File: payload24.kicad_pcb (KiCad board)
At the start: 6 copper layers, 87.1 x 89.4 mm, 21 parts, among them J1 532540370, J2 532540370, J3 460150206, J4 532540370, Q1 CSD19503KCS, Q2 CSD19503KCS, SW1 FingerTech

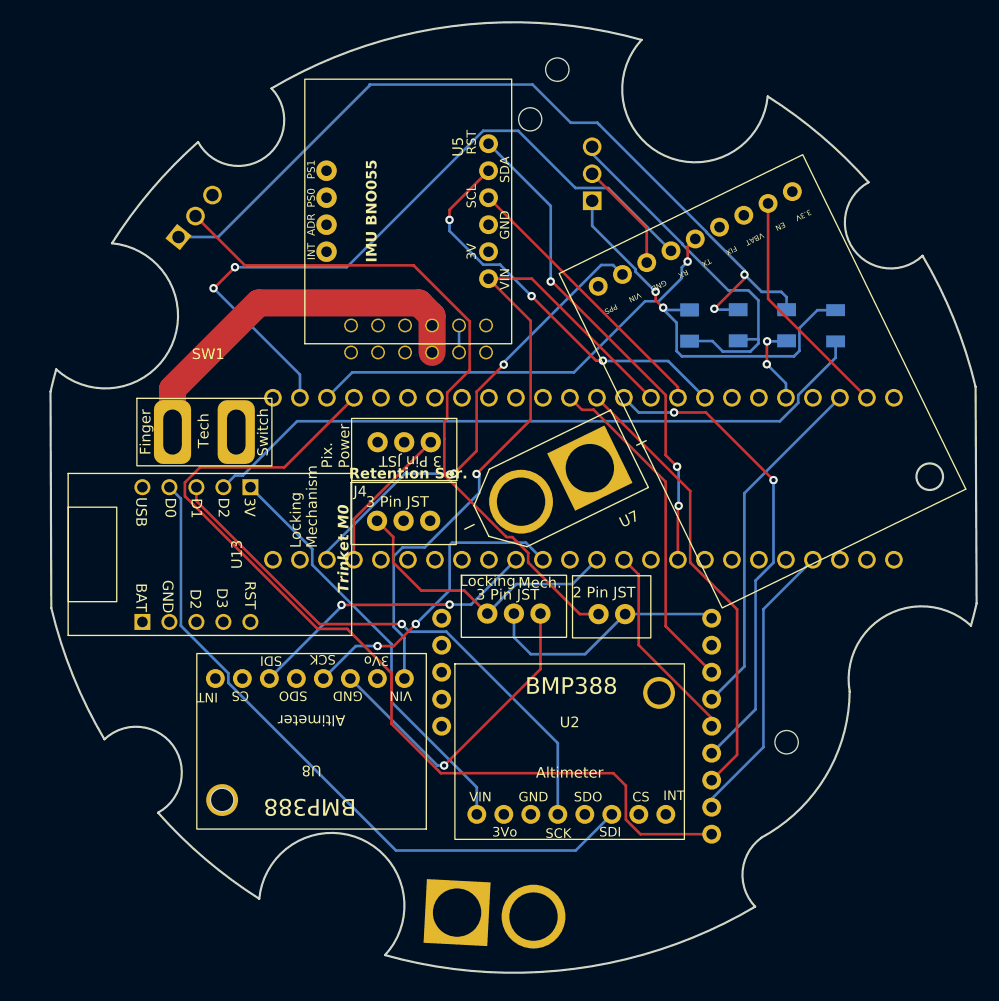
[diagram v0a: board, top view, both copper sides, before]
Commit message: update
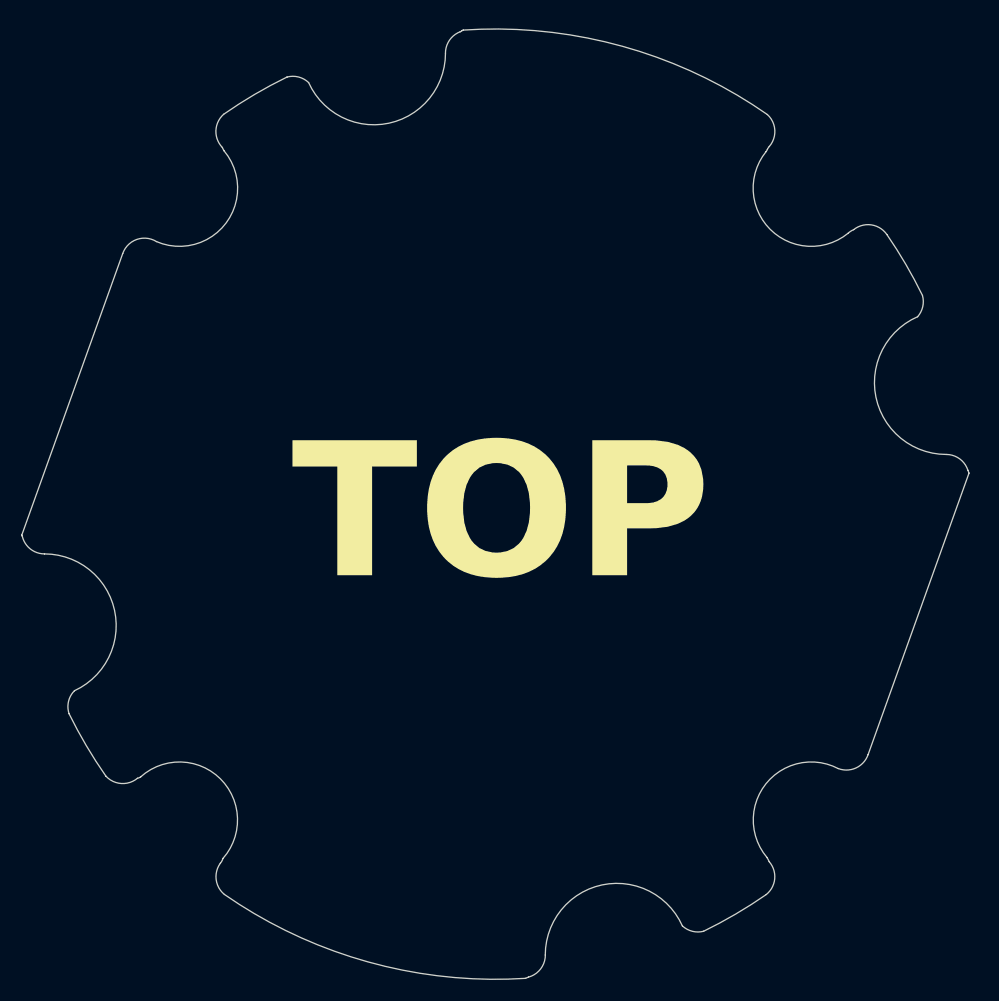
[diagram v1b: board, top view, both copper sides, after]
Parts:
- removed J1, J2, J4: 532540370, JST-XH3:JST-XH3
- removed J3: 460150206, JST-XH2:JST-XH2
- removed Q1, Q2: CSD19503KCS, teensyMosfet:teensyMosfet
- removed R1: 500, 500Ohm:RESC3216X65N
- removed R2: 1000, 1kOhm:RESC3216X70N
- removed R3, R4: 10K, 10KOhm:RESC3216X70N
- removed SW1: FingerTech, FingerTech:FingerTech
- removed U1: ~, Teensy:TEENSY41
- removed U13: ~, Trinket M0:Trinket M0
- removed U14: ~, BNO055:BNO055
- removed U2, U8: ~, BMP388:BMP388
- removed U3: ~, adafruit gps:GPS_adafruit
- removed U4: ~, RFModule:RFM_LoRa
- removed U5: ~, poluluRegulator:VoltageRegulator
- removed U6, U7: ~, XT60:AMASS_XT60-M
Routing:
- net RST3: track 87.9 -> 0.00 mm
- net Net-(Q2-Pad1): track 79.6 -> 0.00 mm, vias 2 -> 0
- net RX1: track 67.5 -> 0.00 mm, vias 2 -> 0
- net 3.3V-Teensy: track 66.4 -> 0.00 mm, vias 1 -> 0
- net GND - NMOS2: track 65.8 -> 0.00 mm
- net SDA3: track 64.7 -> 0.00 mm
- net Power Signal: track 64.6 -> 0.00 mm
- net SCL3: track 51.4 -> 0.00 mm, vias 1 -> 0
- net RST2: track 46.7 -> 0.00 mm, vias 3 -> 0
- net MISO: track 45.4 -> 0.00 mm, vias 2 -> 0
- net 3.3V-Teensy1: track 43.9 -> 0.00 mm, vias 2 -> 0
- net MOSI: track 42.4 -> 0.00 mm
- net TX1: track 42.3 -> 0.00 mm, vias 1 -> 0
- net GND - NMOS1: track 40.7 -> 0.00 mm, vias 1 -> 0
- net 3.3V-Trinket: track 39.6 -> 0.00 mm
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- removed copper zone on In4.Cu, net /22.2V
- removed copper zone on In2.Cu, net 5V-Power Reg.
- removed copper zone on In1.Cu, net GND
- removed copper zone on In3.Cu, net GND - NMOS1
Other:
- board size 87.1 x 89.4 mm -> 89.1 x 89.4 mm
- board text added: "BOTTOM"
- board text added: "TOP"
- board text removed: "Locking"
- board text removed: "Mech."
- board text removed: "Mechanism"
- board text removed: "Pix. Power"
- board text removed: "Retention Ser."

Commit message: PCB laid out
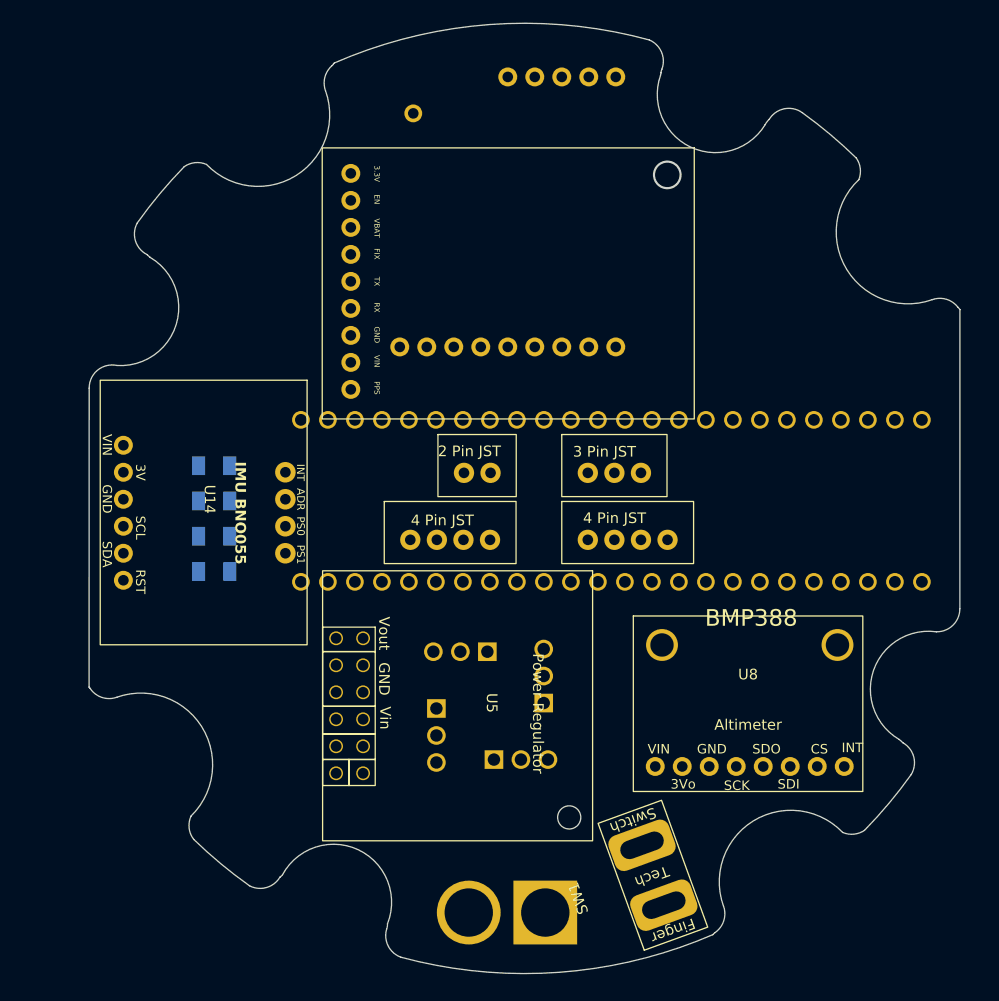
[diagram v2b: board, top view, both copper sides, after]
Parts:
- added J1: JST-XH3, JST-XH3:JST-XH3, F.Cu at (69.2, 54.2)
- added J2: PixHawk, JST-XH2:JST-XH2, F.Cu at (57.5, 54.2)
- added J3: Motors, JST-XH3:JST-XH4, F.Cu at (69.2, 60.5)
- added J4: Motors, JST-XH3:JST-XH4, F.Cu at (52.5, 60.5)
- added Q2: CSD19503KCS, teensyMosfet:teensyMosfet, B.Cu at (59.6, 74.6)
- added Q3: IRLB4132, teensyMosfet:teensyMosfet, B.Cu at (67.5, 76.9)
- added R2: 1000, 1kOhm:RESC3216X70N, B.Cu at (36.5, 57.1)
- added R3: 10K, 10KOhm:RESC3216X70N, B.Cu at (36.5, 60.4)
- added R5: 1000, 1kOhm:RESC3216X70N, B.Cu at (36.5, 63.8)
- added R6: 10K, 10KOhm:RESC3216X70N, B.Cu at (36.5, 67.1)
- added SW1: FingerTech, FingerTech:FingerTech, F.Cu at (76.9, 102.7)
- added U1: ~, Teensy:TEENSY41, B.Cu at (49.7, 52.8)
- added U14: ~, BNO055:BNO055, F.Cu at (35.5, 60.3)
- added U2: LMS1585ACT-3.3/NOPB, teensyMosfet:vRegulator, B.Cu at (65.3, 84.8)
- added U3: ~, adafruit gps:GPS_adafruit, F.Cu at (81.6, 27.2)
- added U4: ~, RFModule:RFM_LoRa, B.Cu at (65.2, 33.4)
- added U5: ~, poluluRegulator:VoltageRegulator, F.Cu at (72.0, 67.0)
- added U6: ~, XT60:AMASS_XT60-M, B.Cu at (64.0, 99.2)
- added U7: LMS1585ACT-3.3/NOPB, teensyMosfet:vRegulator, B.Cu at (57.4, 82.5)
- added U8: ~, BMP388:BMP388, F.Cu at (86.7, 77.2)
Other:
- board size 89.1 x 89.4 mm -> 81.9 x 89.4 mm
- board text removed: "BOTTOM"
- board text removed: "TOP"
